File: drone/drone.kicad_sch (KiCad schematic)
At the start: 52 parts, among them J2 HMC5883, J3 Conn_01x03_Pin, SW1 SW_Push, SW2 SW_Push, U1 ESP32-WROOM-32D, U2 MPU-6050, U3 MP2303ADN

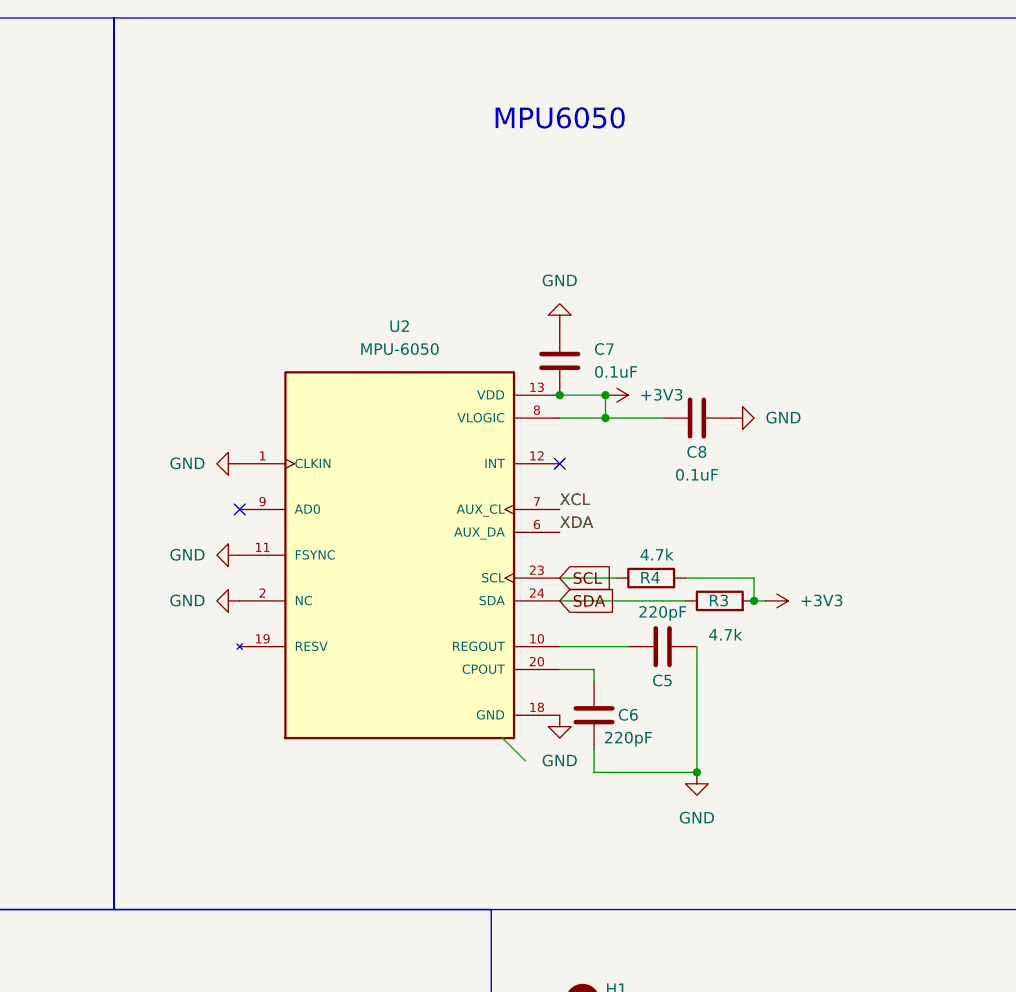
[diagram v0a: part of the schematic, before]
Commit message: hi
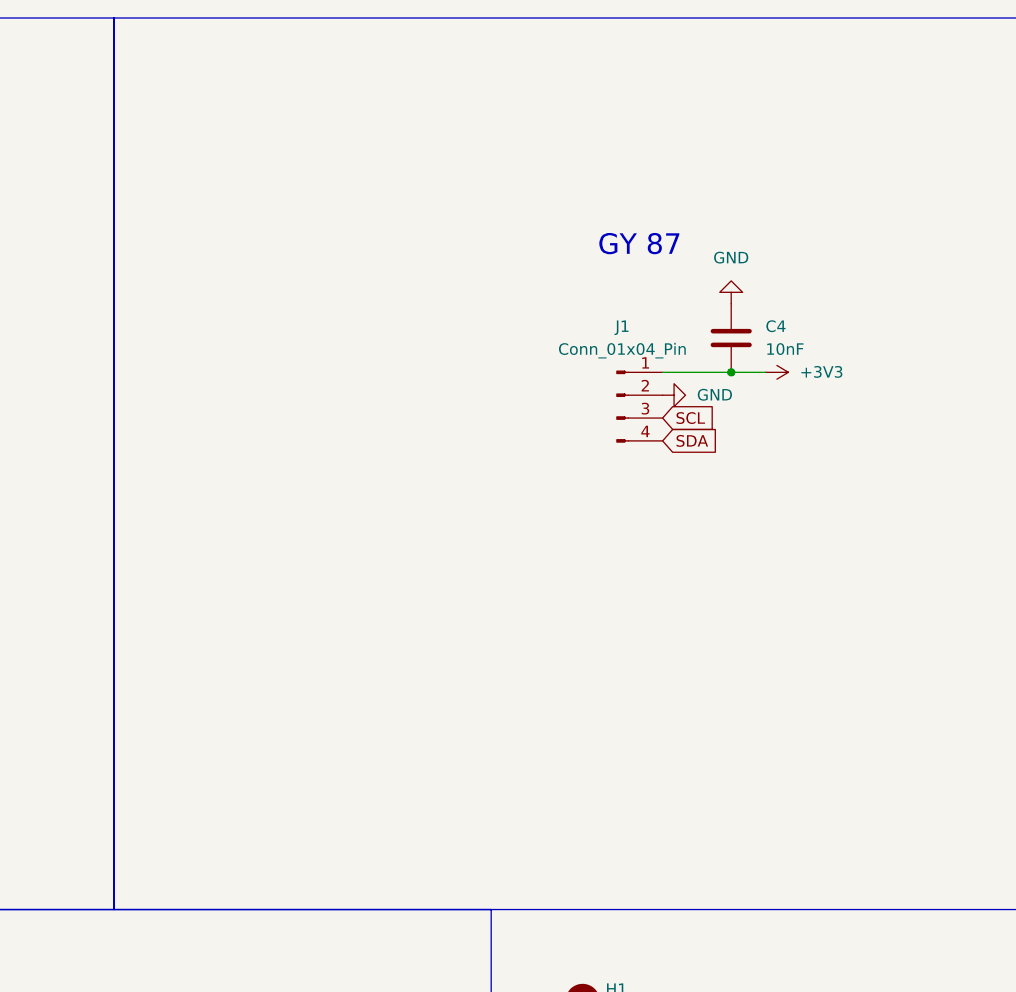
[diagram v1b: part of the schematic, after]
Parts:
- removed C5, C6: 220pF, Capacitor_SMD:C_0805_2012Metric_Pad1.18x1.45mm_HandSolder, symbol Device:C
- removed C7, C8: 0.1uF, Capacitor_SMD:C_0805_2012Metric_Pad1.18x1.45mm_HandSolder, symbol Device:C
- removed R3, R4: 4.7k, Resistor_SMD:R_0805_2012Metric_Pad1.20x1.40mm_HandSolder, symbol Device:R
- removed U2: MPU-6050, MPU-6050:QFN50P400X400X95-24N, symbol MPU-6050:MPU-6050
- added C4: 10nF, Capacitor_SMD:C_0805_2012Metric_Pad1.18x1.45mm_HandSolder, symbol Device:C
- added J1: Conn_01x04_Pin, Connector_PinSocket_2.54mm:PinSocket_1x04_P2.54mm_Vertical, symbol Connector:Conn_01x04_Pin
- H1, H2, H3, H4: footprint MountingHole:MountingHole_3.5mm -> MountingHole:MountingHole_3.2mm_M3
- TP10, TP3, TP4, TP5, TP6, TP7, TP8, TP9: footprint TestPoint:TestPoint_Pad_D2.5mm -> TestPoint:TestPoint_Pad_2.5x2.5mm
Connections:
- net +3V3: now also C4.1, J1.1 (Pin_1)
- net GND: now also C4.2, J1.2 (Pin_2)
- net SCL: now also J1.3 (Pin_3)
- net SDA: now also J1.4 (Pin_4)
- no-connect marks 2 -> 0
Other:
- note added: "GY 87"
- note removed: "MPU6050"
